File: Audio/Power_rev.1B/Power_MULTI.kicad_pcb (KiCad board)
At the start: 2 copper layers, 195.6 x 101.6 mm, 76 parts, among them P1 CONN_01X02, P2 CONN_01X02, P3 CONN_01X02, P4 CONN_01X02, Q1 NPN(TO-220-BCE), Q2 PNP(TO-220-BCE), Q3 NPN(TO-220-BCE), Q4 PNP(TO-220-BCE)

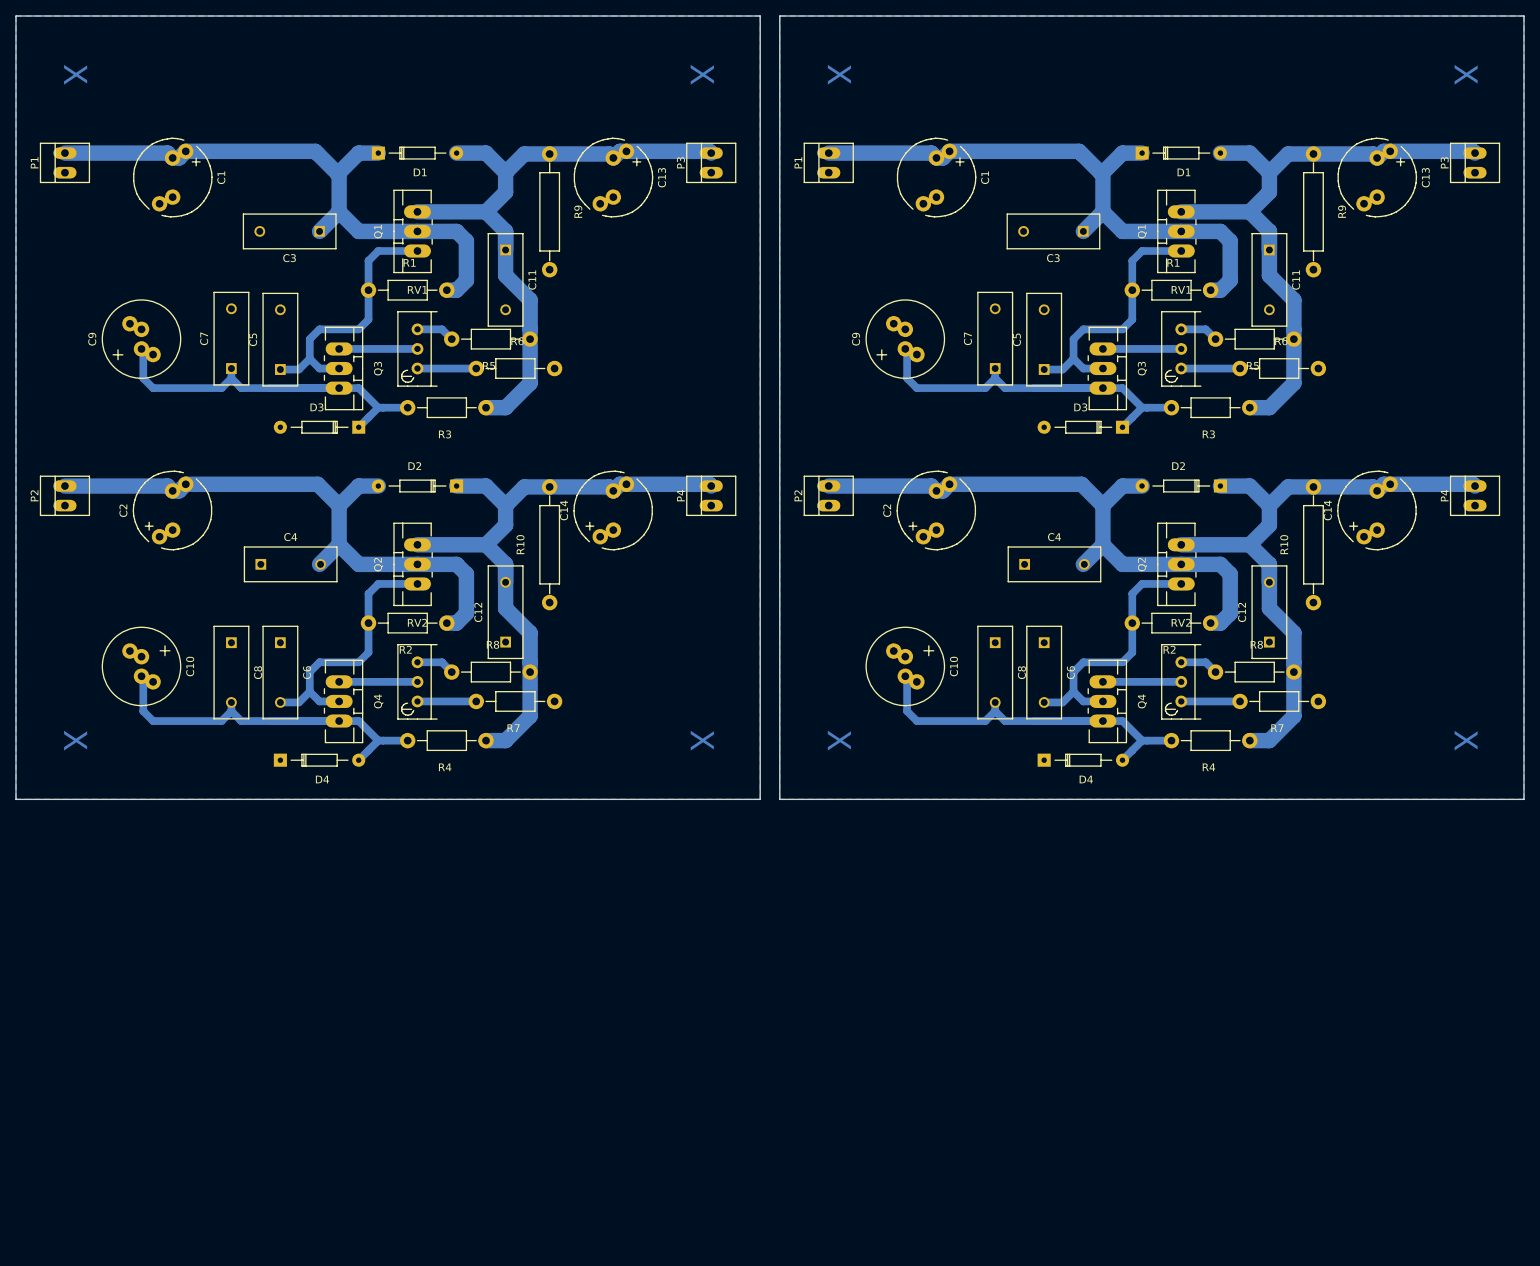
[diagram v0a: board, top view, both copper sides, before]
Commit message: further tweaking(1)
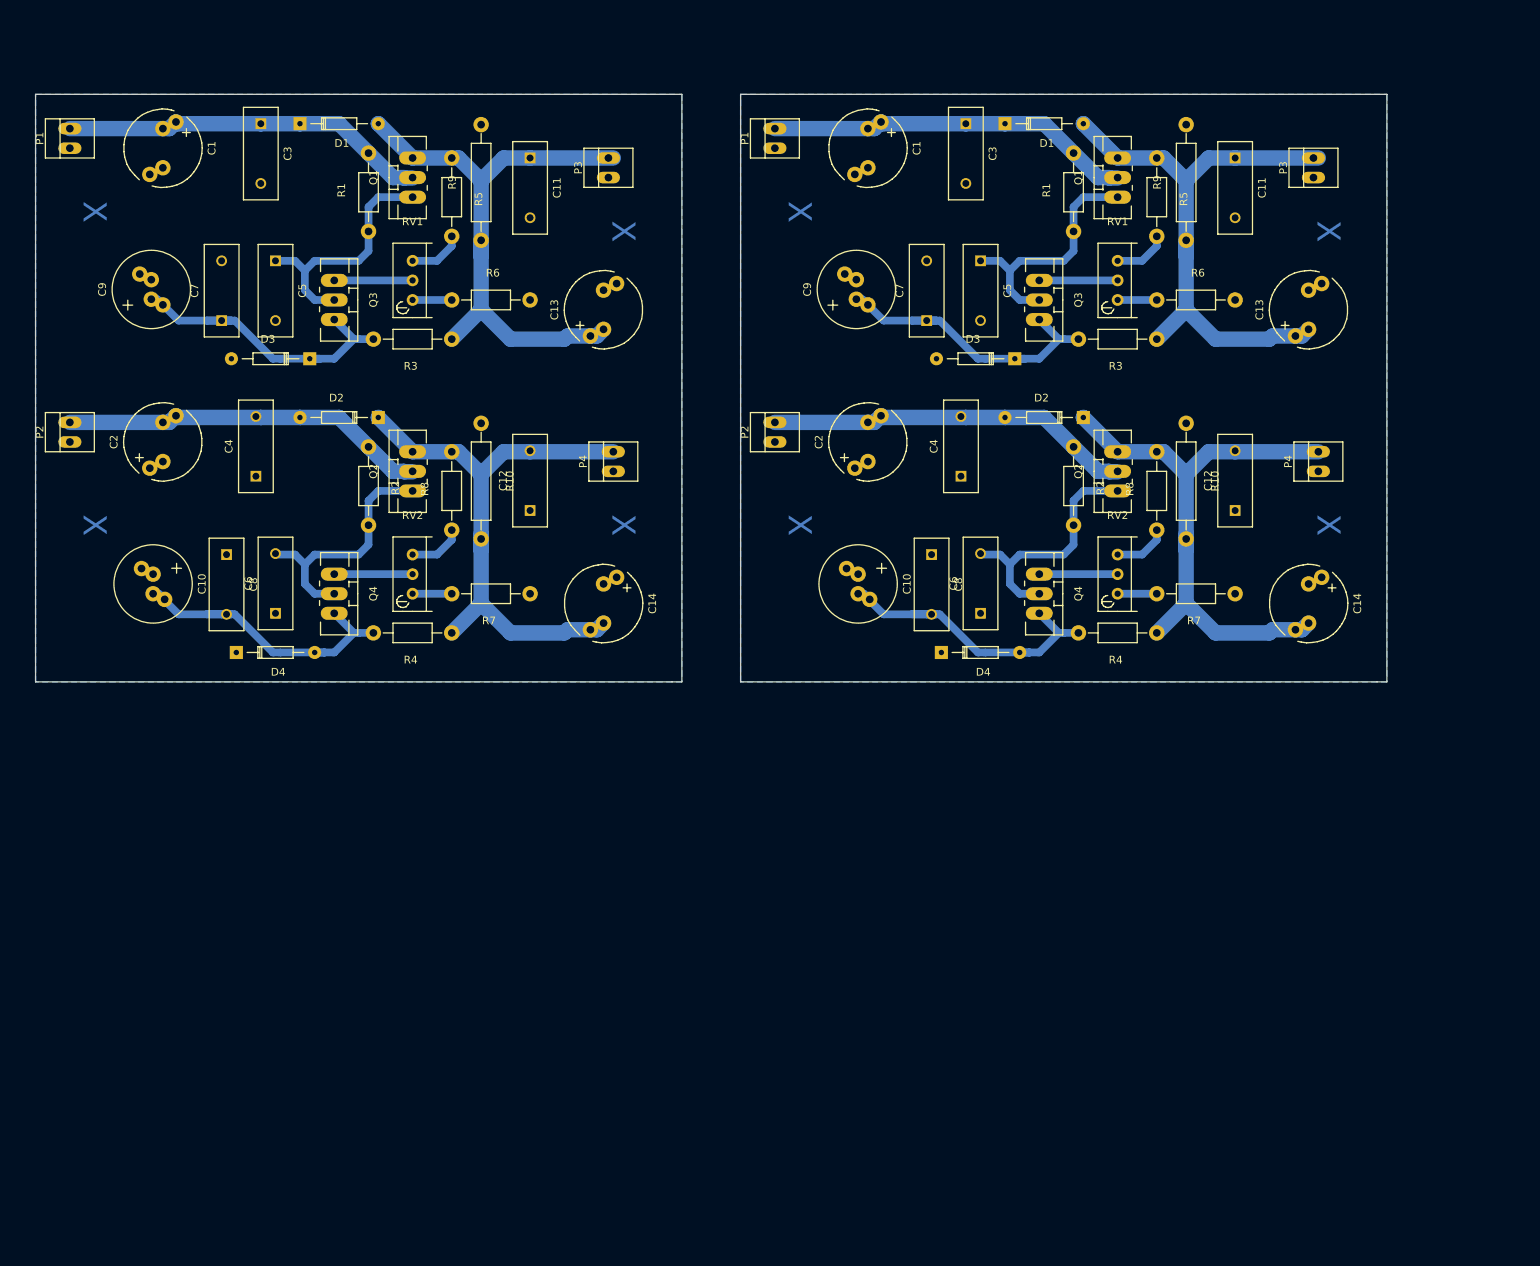
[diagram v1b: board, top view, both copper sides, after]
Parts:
- removed the C1 at (43.2, 41.3)
- removed the C1 at (142.2, 41.3)
- removed the C10 at (39.1, 104.7)
- removed the C10 at (138.2, 104.7)
- removed the C11 at (86.4, 50.7)
- removed the C11 at (185.4, 50.7)
- removed the C12 at (86.4, 101.5)
- removed the C12 at (185.4, 101.5)
- removed the C13 at (100.3, 41.3)
- removed the C13 at (199.4, 41.3)
- removed the C14 at (100.3, 84.5)
- removed the C14 at (199.4, 84.5)
- removed the C2 at (43.2, 84.5)
- removed the C2 at (142.2, 84.5)
- removed the C3 at (62.2, 48.3)
- removed the C3 at (161.3, 48.3)
- removed the C4 at (54.6, 91.4)
- removed the C4 at (153.7, 91.4)
- removed the C5 at (57.1, 66.2)
- removed the C5 at (156.2, 66.2)
- removed the C6 at (57.1, 101.6)
- removed the C6 at (156.2, 101.6)
- removed the C7 at (50.8, 66.0)
- removed the C7 at (149.9, 66.0)
- removed the C8 at (50.8, 101.6)
- removed the C8 at (149.9, 101.6)
- removed the C9 at (39.1, 62.2)
- removed the C9 at (138.2, 62.2)
- removed the D1 at (69.8, 38.1)
- removed the D1 at (168.9, 38.1)
- removed the D2 at (80.0, 81.3)
- removed the D2 at (179.1, 81.3)
- removed the D3 at (67.3, 73.7)
- removed the D3 at (166.4, 73.7)
- removed the D4 at (57.1, 116.8)
- removed the D4 at (156.2, 116.8)
- removed the P1 at (29.2, 39.4)
- removed the P1 at (128.3, 39.4)
- removed the P2 at (29.2, 82.5)
- removed the P2 at (128.3, 82.5)
- removed the P3 at (113.0, 39.4)
- removed the P3 at (212.1, 39.4)
- removed the P4 at (113.0, 82.5)
- removed the P4 at (212.1, 82.5)
- removed the Q1 at (74.9, 48.3)
- removed the Q1 at (174.0, 48.3)
- removed the Q2 at (74.9, 91.4)
- removed the Q2 at (174.0, 91.4)
- removed the Q3 at (64.8, 66.0)
- removed the Q3 at (163.8, 66.0)
- removed the Q4 at (64.8, 109.2)
- removed the Q4 at (163.8, 109.2)
- removed the R1 at (73.7, 55.9)
- removed the R1 at (172.7, 55.9)
- removed the R10 at (92.1, 88.9)
- removed the R10 at (191.1, 88.9)
- removed the R2 at (73.7, 99.1)
- removed the R2 at (172.7, 99.1)
- removed the R3 at (78.7, 71.1)
- removed the R3 at (177.8, 71.1)
- removed the R4 at (78.7, 114.3)
- removed the R4 at (177.8, 114.3)
- removed the R5 at (84.5, 62.2)
- removed the R5 at (183.5, 62.2)
- removed the R6 at (87.6, 66.0)
- removed the R6 at (186.7, 66.0)
- removed the R7 at (87.6, 109.2)
- removed the R7 at (186.7, 109.2)
- removed the R8 at (84.5, 105.4)
- removed the R8 at (183.5, 105.4)
- removed the R9 at (92.1, 45.7)
- removed the R9 at (191.1, 45.7)
- removed the RV1 at (74.9, 66.0)
- removed the RV1 at (174.0, 66.0)
- removed the RV2 at (74.9, 109.2)
- removed the RV2 at (174.0, 109.2)
- added C1: 820uF,100V, Capacitors_ThroughHole:C_Radial_D10_L20_P5-7.5, F.Cu at (41.9, 37.5)
- added C1: 820uF,100V, Capacitors_ThroughHole:C_Radial_D10_L20_P5-7.5, F.Cu at (133.3, 37.5)
- added C10: 22uF,60V+, Capacitors_ThroughHole:C_Radial_D10_L20_P2.5-5, F.Cu at (40.6, 94.0)
- added C10: 22uF,60V+, Capacitors_ThroughHole:C_Radial_D10_L20_P2.5-5, F.Cu at (132.1, 94.0)
- added C11: 0.1uF,60V+, Capacitors_ThroughHole:C_Disc_D12_P7.75, F.Cu at (89.5, 38.7)
- added C11: 0.1uF,60V+, Capacitors_ThroughHole:C_Disc_D12_P7.75, F.Cu at (181.0, 38.7)
- added C12: 0.1uF,60V+, Capacitors_ThroughHole:C_Disc_D12_P7.75, F.Cu at (89.5, 84.5)
- added C12: 0.1uF,60V+, Capacitors_ThroughHole:C_Disc_D12_P7.75, F.Cu at (181.0, 84.5)
- added C13: 470uF,200V, Capacitors_ThroughHole:C_Radial_D10_L20_P5-7.5, F.Cu at (99.1, 58.4)
- added C13: 470uF,200V, Capacitors_ThroughHole:C_Radial_D10_L20_P5-7.5, F.Cu at (190.5, 58.4)
- added C14: 470uF,200V, Capacitors_ThroughHole:C_Radial_D10_L20_P5-7.5, F.Cu at (99.1, 96.5)
- added C14: 470uF,200V, Capacitors_ThroughHole:C_Radial_D10_L20_P5-7.5, F.Cu at (190.5, 96.5)
- added C2: 820uF,100V, Capacitors_ThroughHole:C_Radial_D10_L20_P5-7.5, F.Cu at (41.9, 75.6)
- added C2: 820uF,100V, Capacitors_ThroughHole:C_Radial_D10_L20_P5-7.5, F.Cu at (133.3, 75.6)
- added C3: 0.1uF,125V, Capacitors_ThroughHole:C_Disc_D12_P7.75, F.Cu at (54.6, 34.3)
- added C3: 0.1uF,125V, Capacitors_ThroughHole:C_Disc_D12_P7.75, F.Cu at (146.1, 34.3)
- added C4: 0.1uF,125V, Capacitors_ThroughHole:C_Disc_D12_P7.75, F.Cu at (54.0, 80.0)
- added C4: 0.1uF,125V, Capacitors_ThroughHole:C_Disc_D12_P7.75, F.Cu at (145.4, 80.0)
- added C5: 0.47uF,125V, Capacitors_ThroughHole:C_Disc_D12_P7.75, F.Cu at (56.5, 52.1)
- added C5: 0.47uF,125V, Capacitors_ThroughHole:C_Disc_D12_P7.75, F.Cu at (148.0, 52.1)
- added C6: 0.47uF,125V, Capacitors_ThroughHole:C_Disc_D12_P7.75, F.Cu at (56.5, 97.8)
- added C6: 0.47uF,125V, Capacitors_ThroughHole:C_Disc_D12_P7.75, F.Cu at (148.0, 97.8)
- added C7: 0.1uF,60V+, Capacitors_ThroughHole:C_Disc_D12_P7.75, F.Cu at (49.5, 59.8)
- added C7: 0.1uF,60V+, Capacitors_ThroughHole:C_Disc_D12_P7.75, F.Cu at (141.0, 59.8)
- added C8: 0.1uF,60V+, Capacitors_ThroughHole:C_Disc_D12_P7.75, F.Cu at (50.2, 90.2)
- added C8: 0.1uF,60V+, Capacitors_ThroughHole:C_Disc_D12_P7.75, F.Cu at (141.6, 90.2)
- added C9: 22uF,60V+, Capacitors_ThroughHole:C_Radial_D10_L20_P2.5-5, F.Cu at (40.4, 55.8)
- added C9: 22uF,60V+, Capacitors_ThroughHole:C_Radial_D10_L20_P2.5-5, F.Cu at (131.8, 55.8)
- added D1: D, Diodes_ThroughHole:Diode_DO-35_SOD27_Horizontal_RM10, F.Cu at (59.7, 34.3)
- added D1: D, Diodes_ThroughHole:Diode_DO-35_SOD27_Horizontal_RM10, F.Cu at (151.1, 34.3)
- added D2: D, Diodes_ThroughHole:Diode_DO-35_SOD27_Horizontal_RM10, F.Cu at (69.8, 72.4)
- added D2: D, Diodes_ThroughHole:Diode_DO-35_SOD27_Horizontal_RM10, F.Cu at (161.3, 72.4)
- added D3: ZENER, Diodes_ThroughHole:Diode_DO-35_SOD27_Horizontal_RM10, F.Cu at (61.0, 64.8)
- added D3: ZENER, Diodes_ThroughHole:Diode_DO-35_SOD27_Horizontal_RM10, F.Cu at (152.4, 64.8)
- added D4: ZENER, Diodes_ThroughHole:Diode_DO-35_SOD27_Horizontal_RM10, F.Cu at (51.4, 102.9)
- added D4: ZENER, Diodes_ThroughHole:Diode_DO-35_SOD27_Horizontal_RM10, F.Cu at (142.9, 102.9)
- added P1: CONN_01X02, Connect:PINHEAD1-2, F.Cu at (29.8, 36.2)
- added P1: CONN_01X02, Connect:PINHEAD1-2, F.Cu at (121.3, 36.2)
- added P2: CONN_01X02, Connect:PINHEAD1-2, F.Cu at (29.8, 74.3)
- added P2: CONN_01X02, Connect:PINHEAD1-2, F.Cu at (121.3, 74.3)
- added P3: CONN_01X02, Connect:PINHEAD1-2, F.Cu at (99.7, 40.0)
- added P3: CONN_01X02, Connect:PINHEAD1-2, F.Cu at (191.1, 40.0)
- added P4: CONN_01X02, Connect:PINHEAD1-2, F.Cu at (100.3, 78.1)
- added P4: CONN_01X02, Connect:PINHEAD1-2, F.Cu at (191.8, 78.1)
- added Q1: NPN(TO-220-BCE), TO_SOT_Packages_THT:TO-220_Neutral123_Vertical_LargePads, F.Cu at (74.3, 41.3)
- added Q1: NPN(TO-220-BCE), TO_SOT_Packages_THT:TO-220_Neutral123_Vertical_LargePads, F.Cu at (165.7, 41.3)
- added Q2: PNP(TO-220-BCE), TO_SOT_Packages_THT:TO-220_Neutral123_Vertical_LargePads, F.Cu at (74.3, 79.4)
- added Q2: PNP(TO-220-BCE), TO_SOT_Packages_THT:TO-220_Neutral123_Vertical_LargePads, F.Cu at (165.7, 79.4)
- added Q3: NPN(TO-220-BCE), TO_SOT_Packages_THT:TO-220_Neutral123_Vertical_LargePads, F.Cu at (64.1, 57.1)
- added Q3: NPN(TO-220-BCE), TO_SOT_Packages_THT:TO-220_Neutral123_Vertical_LargePads, F.Cu at (155.6, 57.1)
- added Q4: PNP(TO-220-BCE), TO_SOT_Packages_THT:TO-220_Neutral123_Vertical_LargePads, F.Cu at (64.1, 95.2)
- added Q4: PNP(TO-220-BCE), TO_SOT_Packages_THT:TO-220_Neutral123_Vertical_LargePads, F.Cu at (155.6, 95.2)
- added R1: 18k, Resistors_ThroughHole:Resistor_Horizontal_RM10mm, F.Cu at (68.6, 43.2)
- added R1: 18k, Resistors_ThroughHole:Resistor_Horizontal_RM10mm, F.Cu at (160.0, 43.2)
- added R10: 8.2k,0.5W+, Resistors_ThroughHole:Resistor_Horizontal_RM15mm, F.Cu at (83.2, 80.6)
- added R10: 8.2k,0.5W+, Resistors_ThroughHole:Resistor_Horizontal_RM15mm, F.Cu at (174.6, 80.6)
- added R2: 18k, Resistors_ThroughHole:Resistor_Horizontal_RM10mm, F.Cu at (68.6, 81.3)
- added R2: 18k, Resistors_ThroughHole:Resistor_Horizontal_RM10mm, F.Cu at (160.0, 81.3)
- added R3: 4.3k, Resistors_ThroughHole:Resistor_Horizontal_RM10mm, F.Cu at (74.3, 62.2)
- added R3: 4.3k, Resistors_ThroughHole:Resistor_Horizontal_RM10mm, F.Cu at (165.7, 62.2)
- added R4: 4.3k, Resistors_ThroughHole:Resistor_Horizontal_RM10mm, F.Cu at (74.3, 100.3)
- added R4: 4.3k, Resistors_ThroughHole:Resistor_Horizontal_RM10mm, F.Cu at (165.7, 100.3)
- added R5: 20k, Resistors_ThroughHole:Resistor_Horizontal_RM10mm, F.Cu at (79.4, 43.8)
- added R5: 20k, Resistors_ThroughHole:Resistor_Horizontal_RM10mm, F.Cu at (170.8, 43.8)
- added R6: 27k, Resistors_ThroughHole:Resistor_Horizontal_RM10mm, F.Cu at (84.5, 57.1)
- added R6: 27k, Resistors_ThroughHole:Resistor_Horizontal_RM10mm, F.Cu at (175.9, 57.1)
- added R7: 27k, Resistors_ThroughHole:Resistor_Horizontal_RM10mm, F.Cu at (84.5, 95.2)
- added R7: 27k, Resistors_ThroughHole:Resistor_Horizontal_RM10mm, F.Cu at (175.9, 95.2)
- added R8: 20k, Resistors_ThroughHole:Resistor_Horizontal_RM10mm, F.Cu at (79.4, 81.9)
- added R8: 20k, Resistors_ThroughHole:Resistor_Horizontal_RM10mm, F.Cu at (170.8, 81.9)
- added R9: 8.2k,0.5W+, Resistors_ThroughHole:Resistor_Horizontal_RM15mm, F.Cu at (83.2, 41.9)
- added R9: 8.2k,0.5W+, Resistors_ThroughHole:Resistor_Horizontal_RM15mm, F.Cu at (174.6, 41.9)
- added RV1: 10k, Potentiometers:Potentiometer_Bourns_3296W_3-8Zoll_Inline_ScrewUp, F.Cu at (74.3, 57.1)
- added RV1: 10k, Potentiometers:Potentiometer_Bourns_3296W_3-8Zoll_Inline_ScrewUp, F.Cu at (165.7, 57.1)
- added RV2: 10k, Potentiometers:Potentiometer_Bourns_3296W_3-8Zoll_Inline_ScrewUp, F.Cu at (74.3, 95.2)
- added RV2: 10k, Potentiometers:Potentiometer_Bourns_3296W_3-8Zoll_Inline_ScrewUp, F.Cu at (165.7, 95.2)
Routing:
- net 63-75V(+): track 156.7 -> 95.6 mm
- net 63-75V(-): track 156.7 -> 95.6 mm
- net Net-(C10-Pad2): track 109.0 -> 84.7 mm
- net Net-(C7-Pad1): track 109.0 -> 84.7 mm
- net VCC: track 169.6 -> 153.9 mm
- net VEE: track 169.4 -> 153.9 mm
- net Net-(R7-Pad2): track 15.2 -> 10.2 mm
- net Net-(R6-Pad1): track 15.2 -> 10.2 mm
- net Net-(R8-Pad1): track 9.94 -> 14.3 mm
- net Net-(R5-Pad2): track 9.94 -> 14.3 mm
- net Net-(C5-Pad1): track 68.9 -> 65.0 mm
- net Net-(C6-Pad2): track 68.9 -> 65.0 mm
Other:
- board size 195.6 x 101.6 mm -> 175.3 x 76.2 mm
